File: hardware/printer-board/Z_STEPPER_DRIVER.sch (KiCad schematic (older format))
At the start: 9 parts, among them J7 MS_SELECT, J8 Z, U5 A4988_MODULE

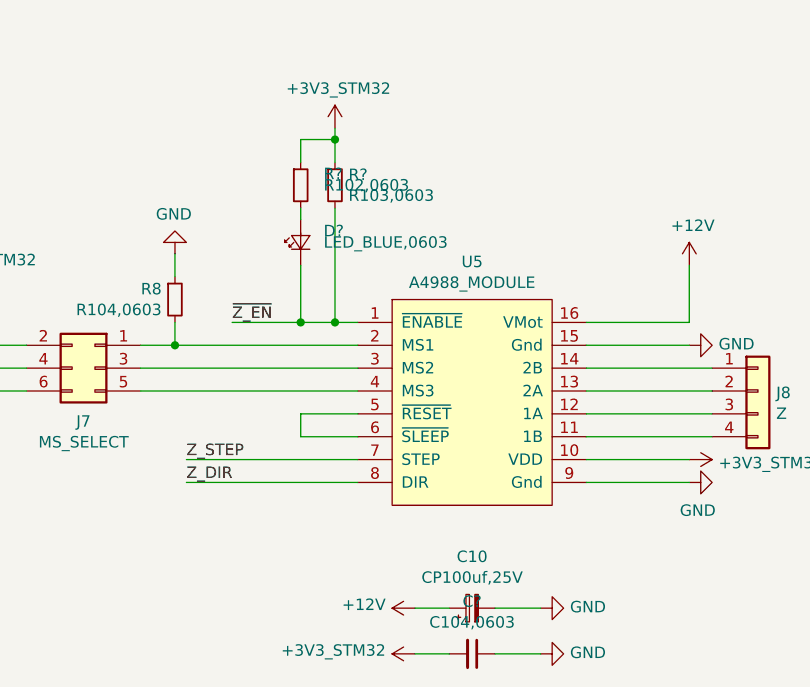
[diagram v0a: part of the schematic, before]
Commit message: update annotations,
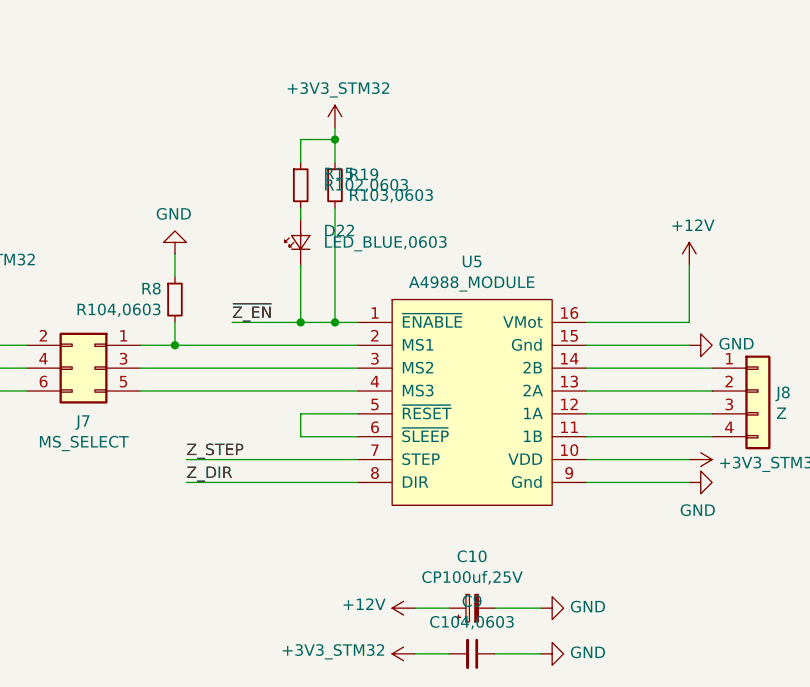
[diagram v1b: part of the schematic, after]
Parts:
- gave numbers to parts that had none: 4
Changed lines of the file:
@@
 $EndBitmap
 $Comp
-L taobao-components:+3V3_STM32 #PWR?
+L taobao-components:+3V3_STM32 #PWR015
 U 1 1 5CC40B36
 P 3500 2700
-F 0 "#PWR?" H 3500 2550 50  0001 C CNN
+F 0 "#PWR015" H 3500 2550 50  0001 C CNN
 F 1 "+3V3_STM32" H 3515 2873 50  0000 C CNN
 F 2 "" H 3500 2700 50  0001 C CNN
@@
 $EndComp
 $Comp
-L taobao-components:+3V3_STM32 #PWR?
+L taobao-components:+3V3_STM32 #PWR017
 U 1 1 5CC40B4D
 P 5400 4250
-F 0 "#PWR?" H 5400 4100 50  0001 C CNN
+F 0 "#PWR017" H 5400 4100 50  0001 C CNN
 F 1 "+3V3_STM32" V 5415 4378 50  0000 L CNN
 F 2 "" H 5400 4250 50  0001 C CNN
@@
 $EndComp
 $Comp
-L taobao-c:C104,0603 C?
+L taobao-c:C104,0603 C9
 U 1 1 5CC40BE7
 P 5650 4250
-F 0 "C?" V 5421 4250 50  0000 C CNN
+F 0 "C9" V 5421 4250 50  0000 C CNN
 F 1 "C104,0603" V 5512 4250 50  0000 C CNN
 F 2 "Capacitor_SMD:C_0603_1608Metric_Pad1.05x0.95mm_HandSolder" H 5650 4250 50  0001 C CNN
@@
 $EndComp
 $Comp
-L taobao-components:+3V3_STM32 #PWR?
+L taobao-components:+3V3_STM32 #PWR016
 U 1 1 5CC40CCA
 P 6600 3400
-F 0 "#PWR?" H 6600 3250 50  0001 C CNN
+F 0 "#PWR016" H 6600 3250 50  0001 C CNN
 F 1 "+3V3_STM32" V 6615 3528 50  0000 L CNN
 F 2 "" H 6600 3400 50  0001 C CNN
@@
 AR Path="/5CC049BB/5CC57FC6" Ref="R?"  Part="1"
 AR Path="/5CC0A4B9/5CC57FC6" Ref="R?"  Part="1"
-AR Path="/5CC0A53C/5CC57FC6" Ref="R?"  Part="1"
+AR Path="/5CC0A53C/5CC57FC6" Ref="R19"  Part="1"
 AR Path="/5CC0A8C5/5CC57FC6" Ref="R?"  Part="1"
 AR Path="/5CC0A8CA/5CC57FC6" Ref="R?"  Part="1"
 AR Path="/5CC0A8CF/5CC57FC6" Ref="R?"  Part="1"
 AR Path="/5CC0AEC9/5CC57FC6" Ref="R?"  Part="1"
-F 0 "R?" H 5109 2246 50  0000 L CNN
+F 0 "R19" H 5109 2246 50  0000 L CNN
 F 1 "R103,0603" H 5109 2155 50  0000 L CNN
 F 2 "Resistor_SMD:R_0603_1608Metric_Pad1.05x0.95mm_HandSolder" H 5050 2200 50  0001 C CNN
@@
 P 5050 1950
 AR Path="/5CC0AEC9/5CC57FCE" Ref="#PWR?"  Part="1"
-AR Path="/5CC0A53C/5CC57FCE" Ref="#PWR?"  Part="1"
-F 0 "#PWR?" H 5050 1800 50  0001 C CNN
+AR Path="/5CC0A53C/5CC57FCE" Ref="#PWR014"  Part="1"
+F 0 "#PWR014" H 5050 1800 50  0001 C CNN
 F 1 "+3V3_STM32" H 5065 2123 50  0000 C CNN
 F 2 "" H 5050 1950 50  0001 C CNN
@@
 AR Path="/5CC15C35/5CC57FD4" Ref="R?"  Part="1"
 AR Path="/5CC0AEC9/5CC57FD4" Ref="R?"  Part="1"
-AR Path="/5CC0A53C/5CC57FD4" Ref="R?"  Part="1"
-F 0 "R?" H 5000 2250 50  0000 L CNN
+AR Path="/5CC0A53C/5CC57FD4" Ref="R15"  Part="1"
+F 0 "R15" H 5000 2250 50  0000 L CNN
 F 1 "R102,0603" H 5000 2200 50  0000 L CNN
 F 2 "Resistor_SMD:R_0603_1608Metric_Pad1.05x0.95mm_HandSolder" H 4900 2200 50  0001 C CNN
@@
 AR Path="/5CC15C35/5CC57FDB" Ref="D?"  Part="1"
 AR Path="/5CC0AEC9/5CC57FDB" Ref="D?"  Part="1"
-AR Path="/5CC0A53C/5CC57FDB" Ref="D?"  Part="1"
-F 0 "D?" V 4950 2350 50  0000 R CNN
+AR Path="/5CC0A53C/5CC57FDB" Ref="D22"  Part="1"
+F 0 "D22" V 4950 2350 50  0000 R CNN
 F 1 "LED_BLUE,0603" V 4900 2350 50  0000 R CNN
 F 2 "LED_SMD:LED_0603_1608Metric_Pad1.05x0.95mm_HandSolder" V 4900 2450 50  0001 C CNN
